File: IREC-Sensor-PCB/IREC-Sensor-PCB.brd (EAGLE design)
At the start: 65 x 56.5 mm, 9 parts, among them J1 RASPBERRYPI-40-PIN-GPIO_PTH_N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, J2 BME280-I2C, J3 BME280-SPI, J4 MPU6050

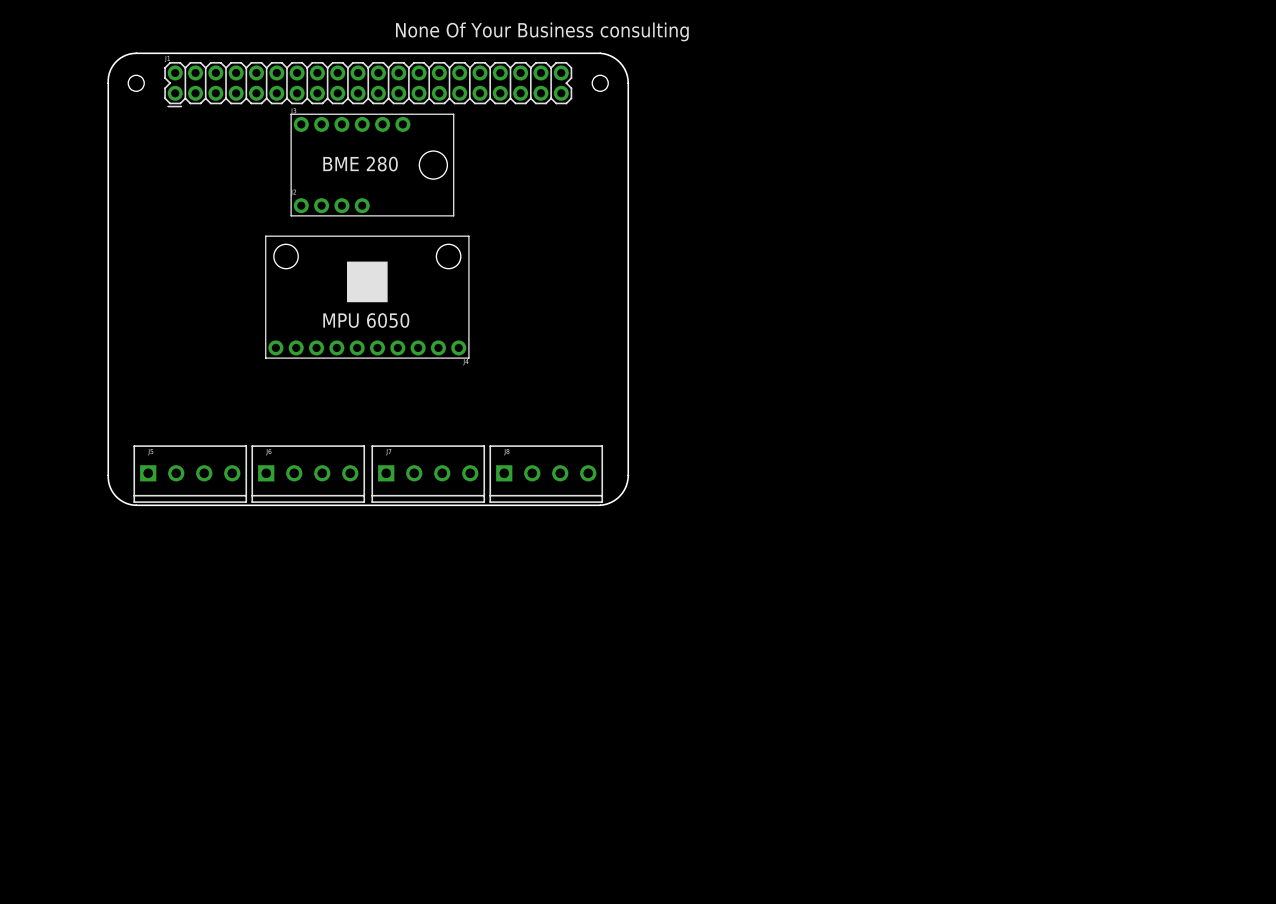
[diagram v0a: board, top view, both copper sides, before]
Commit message: Updated Sensor PCB files
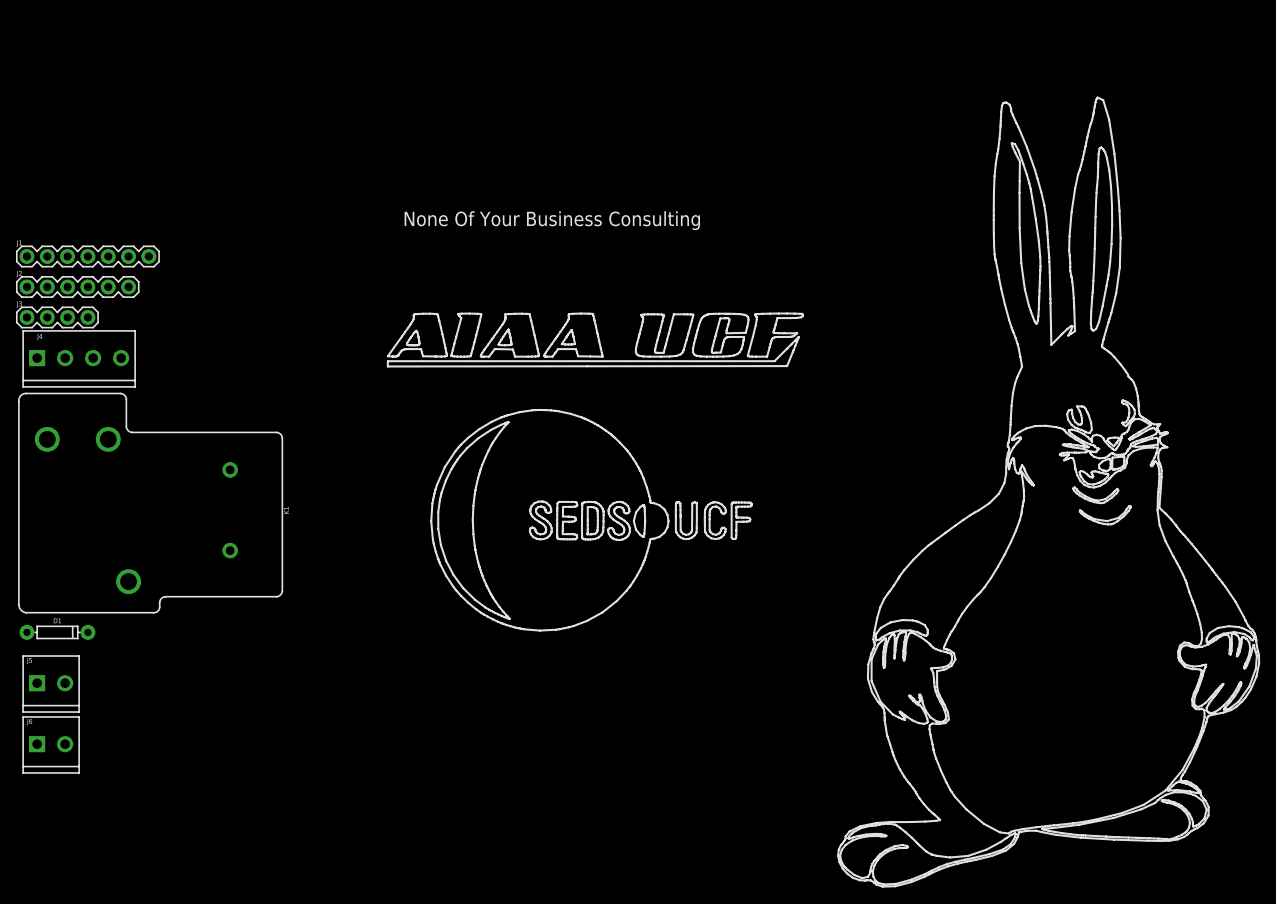
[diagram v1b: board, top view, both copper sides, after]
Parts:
- removed J7, J8: (no value), SparkFun-Connectors:SCREWTERMINAL-3.5MM-4
- added D1: 200mA/100V/1V, SparkFun-DiscreteSemi:DIODE-1N4148
- added K1: RELAY-SPDT-JQX-15F, SparkFun-Electromechanical:RELAY-T90
- J1: value RASPBERRYPI-40-PIN-GPIO_PTH_NO_SHROUD -> (none); device SparkFun-Connectors:2X20 -> SparkFun-Connectors:1X07
- J2: value BME280-I2C -> (none); device SparkFun-Connectors:1X04_NO_SILK -> SparkFun-Connectors:1X06
- J3: value BME280-SPI -> (none); device SparkFun-Connectors:1X06_NO_SILK -> SparkFun-Connectors:1X04
- J4: value MPU6050 -> (none); device SparkFun-Connectors:1X10_NO_SILK -> SparkFun-Connectors:SCREWTERMINAL-3.5MM-4
- J5, J6: device SparkFun-Connectors:SCREWTERMINAL-3.5MM-4 -> SparkFun-Connectors:SCREWTERMINAL-3.5MM-2
- moved J4 52.7 mm to (-8.89, -38.1), turned to 0 degrees
- moved J6 44.3 mm to (-8.89, -86.4)
- moved J3 41.9 mm to (-10.2, -33.0)
- moved J2 35.8 mm to (-10.2, -29.2)
- moved J5 29.7 mm to (-8.89, -78.7)
- moved J1 27.6 mm to (-10.2, -25.4)
- moved FRAME1 23.6 mm to (8.89, -21.6)
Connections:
- removed net VDD: J1.1, J2.2, J4.1
- new net AD_AGM: J3.4
- new net AD_HPT: J1.5
- new net CS_HPT: J1.7
- new net INT: J3.3
- new net N$1: D1.A, J5.2, K1.COIL2
- new net N$2: D1.C, J5.1, K1.COIL1
- new net N$3: J6.2, K1.NO
- new net N$4: J6.1, K1.MAIN
- new net PS0: J3.1
- new net PS1: J3.2
- new net RST: J2.6
- net 3.3V: now also J1.2, J2.2; no longer J1.17
- net 5V: now also J1.1, J2.1, J4.2; no longer J1.2, J1.4
- net GND: now also J1.3, J2.3, J4.1; no longer J1.14, J1.20, J1.25, J1.30, J1.34, J1.39, J1.6, J1.9, J2.1, J4.2
- net SCL: now also J1.4, J2.5, J4.4; no longer J1.5, J2.4, J4.5
- net SDA: now also J1.6, J2.4, J4.3; no longer J1.3, J2.3, J4.6
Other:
- board outline removed
- board text added: "None Of Your Business Consulting"
- board text removed: "BME 280"
- board text removed: "MPU 6050"
- board text removed: "None Of Your Business consulting"
